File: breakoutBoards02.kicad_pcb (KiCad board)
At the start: 2 copper layers, 50 x 50 mm, 45 parts, among them J1 USB_2, M1 Mounting Hole (0.125"), M2 Mounting Hole (0.125"), M3 Mounting Hole (0.125"), M4 Mounting Hole (0.125"), P1 CONN_12, P2 CONN_12, U1 EEPROM_SPI, U2 FT232H, X1 12MHz

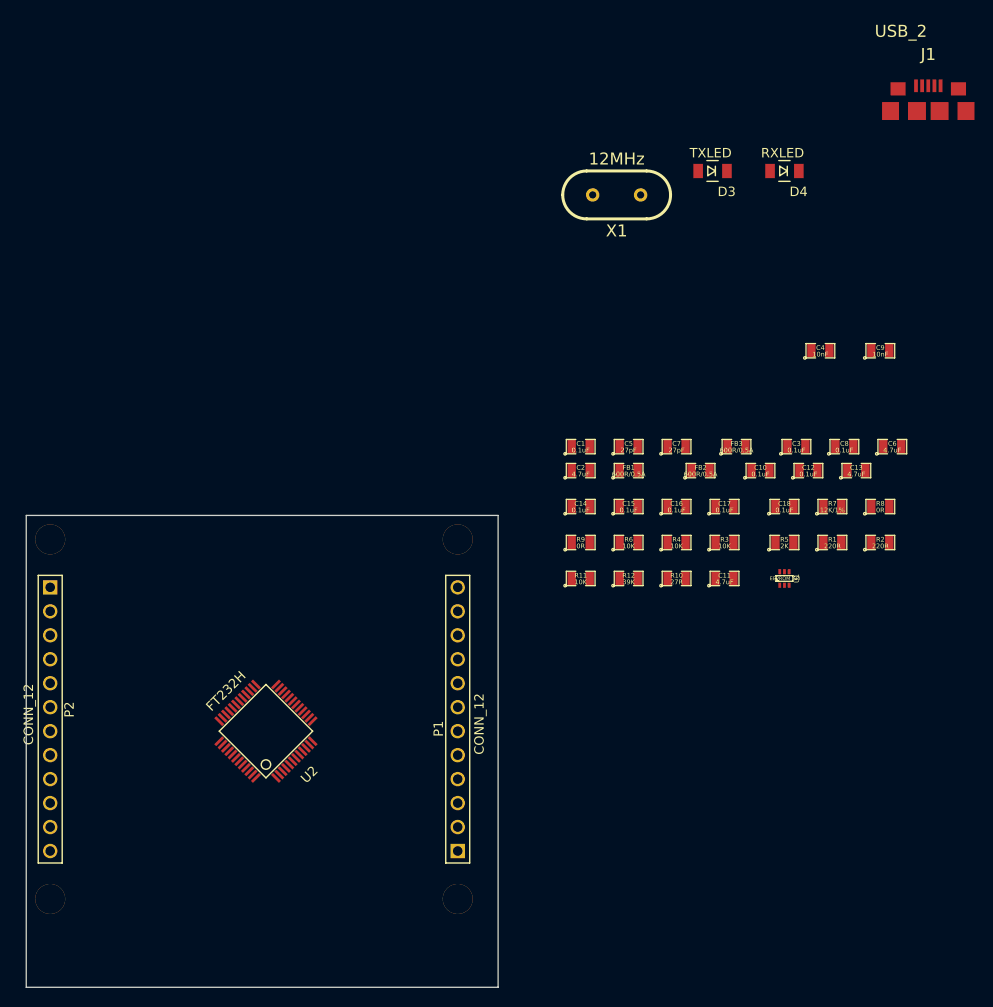
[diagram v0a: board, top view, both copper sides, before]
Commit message: initial layout
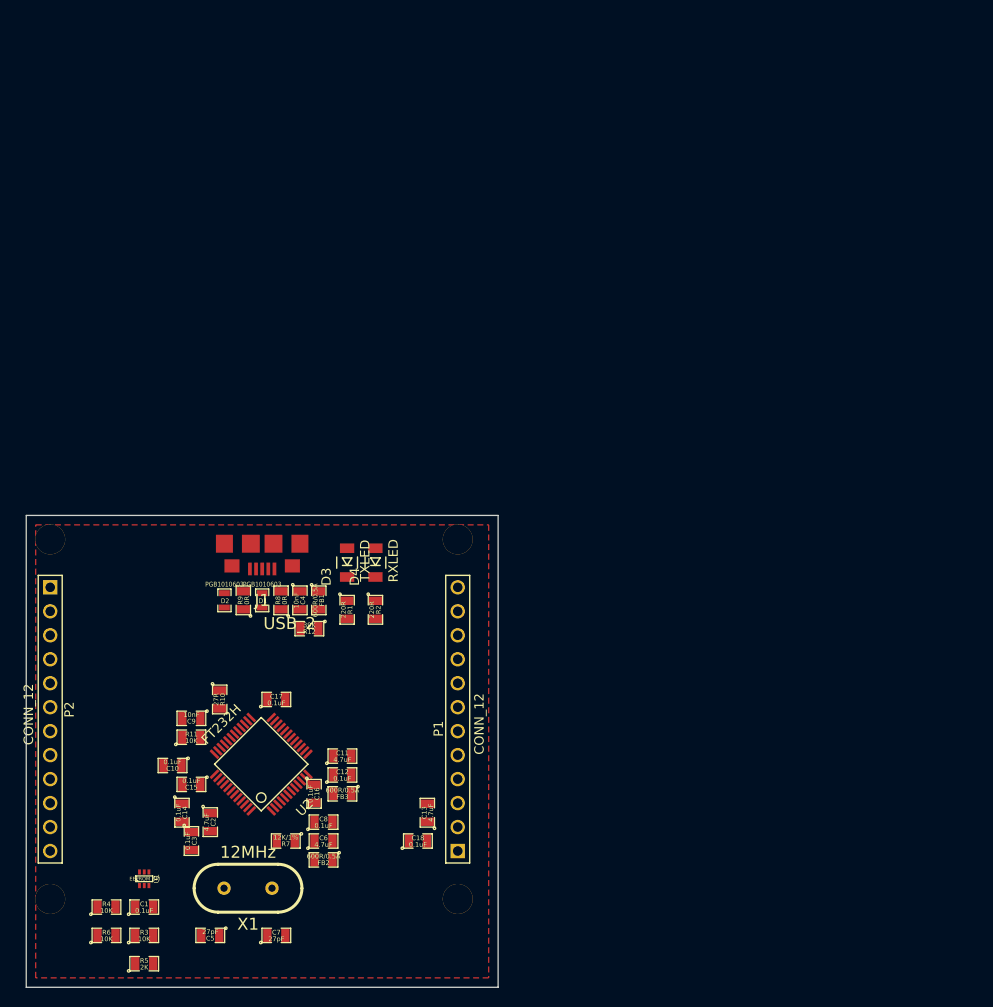
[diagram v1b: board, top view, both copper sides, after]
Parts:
- added D1: PGB1010603, SM0603_Resistor, F.Cu at (125.0, 109.0)
- added D2: PGB1010603, SM0603_Resistor, F.Cu at (121.0, 109.0)
- moved J1 84.2 mm to (125.0, 103.0), turned to 180 degrees
- moved X1 83.2 mm to (123.5, 139.5)
- moved C9 82.7 mm to (117.5, 121.5), turned to 180 degrees
- moved R5 81.2 mm to (112.5, 147.5)
- moved C3 76.5 mm to (117.5, 134.5), turned to 270 degrees
- moved U1 74.9 mm to (112.5, 138.5)
- moved R3 74.3 mm to (112.5, 144.5)
- moved C6 73.3 mm to (131.5, 134.5)
- moved R4 71.7 mm to (108.5, 141.5)
- moved C10 69.7 mm to (115.5, 126.5), turned to 180 degrees
- moved R6 69.2 mm to (108.5, 144.5)
- moved C5 68.2 mm to (119.5, 144.5), turned to 180 degrees
- moved C8 68.0 mm to (131.5, 132.5)
- moved R7 67.9 mm to (127.5, 134.5), turned to 180 degrees
- moved C1 67.2 mm to (112.5, 141.5)
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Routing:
- added copper zone on F.Cu, net GND

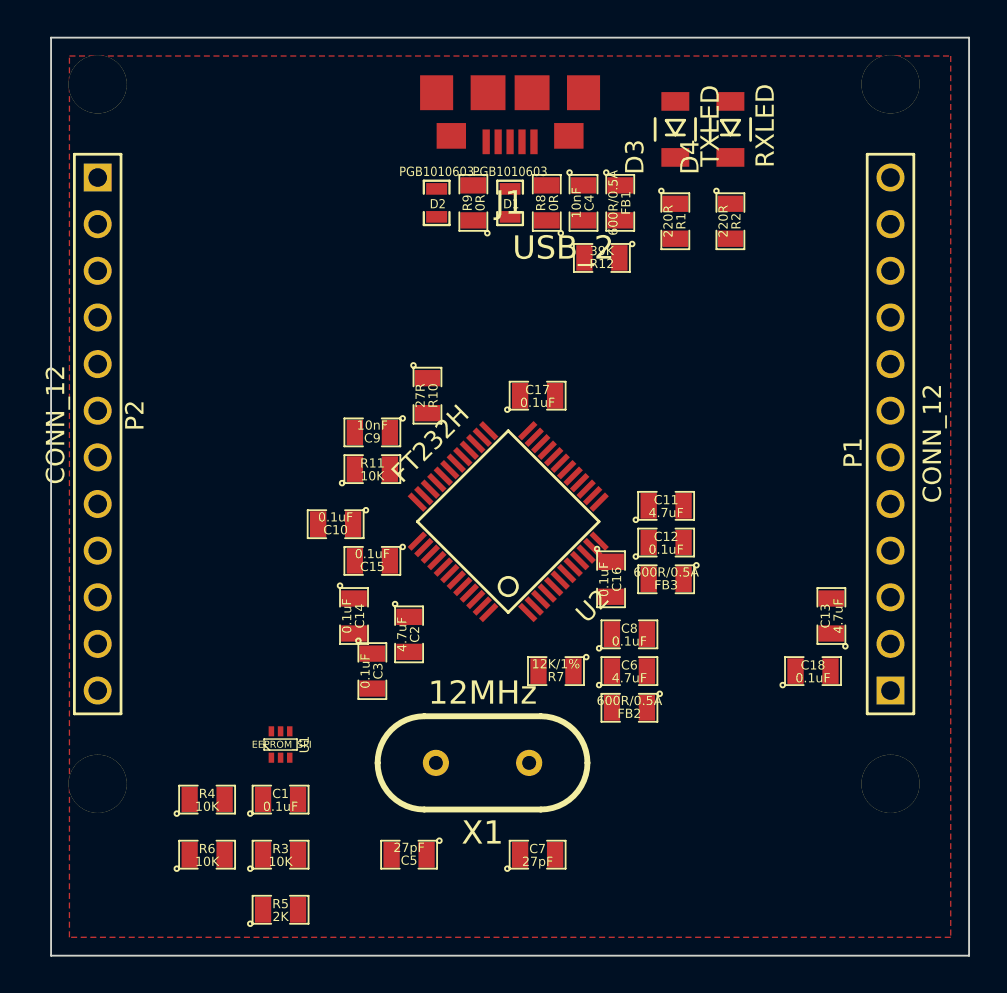
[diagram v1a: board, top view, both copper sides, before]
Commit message: boards
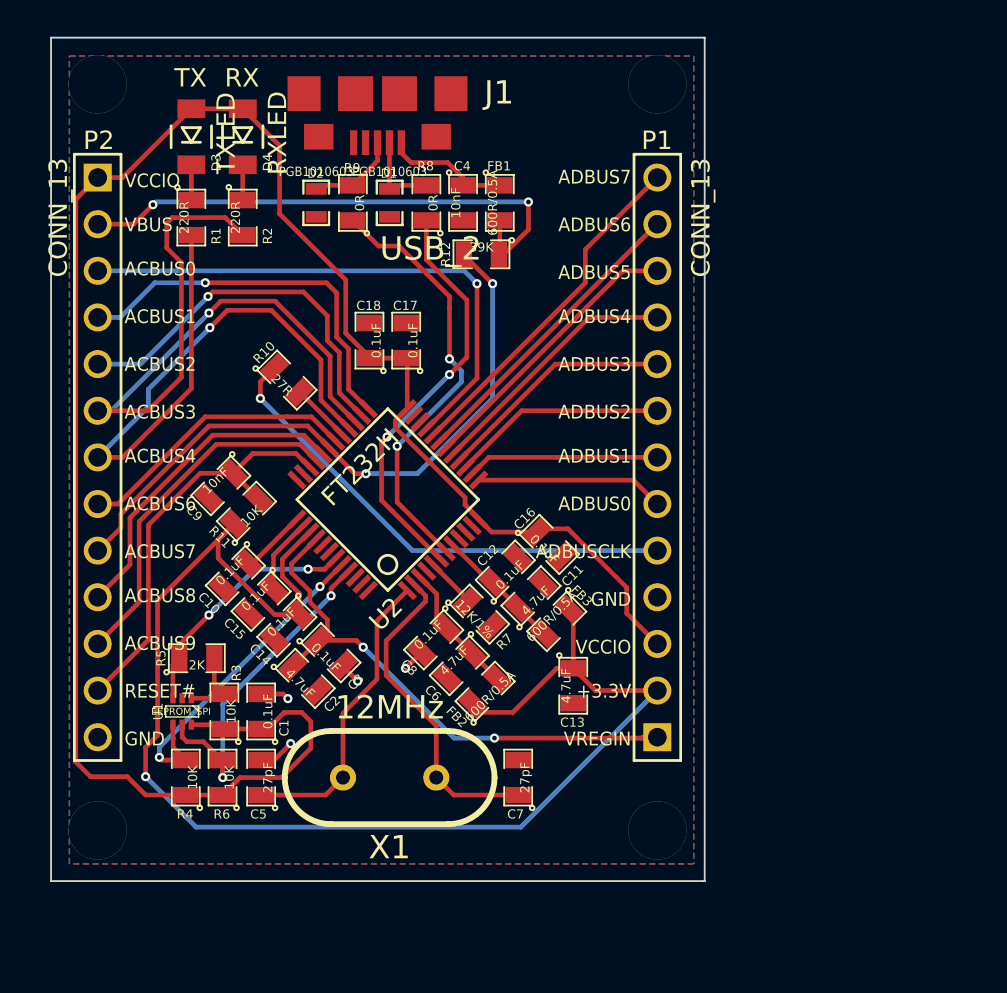
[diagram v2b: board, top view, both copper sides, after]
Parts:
- P1, P2: value CONN_12 -> CONN_13; footprint PIN_ARRAY_12X1 -> PIN_ARRAY_13X1
- moved C18 30.1 mm to (117.3, 116.5), turned to 90 degrees
- moved D4 26.6 mm to (110.4, 105.4)
- moved R2 26.6 mm to (110.4, 109.8)
- moved D3 26.4 mm to (107.6, 105.4)
- moved R1 26.4 mm to (107.6, 109.8)
- moved C13 14.6 mm to (128.4, 135.3), turned to 270 degrees
- moved R5 14.4 mm to (107.9, 133.8)
- moved M1 13.0 mm to (133.0, 143.2)
- moved P1 13.0 mm to (133.0, 125.4)
- moved M4 12.7 mm to (133.0, 102.5)
- moved C8 10.7 mm to (120.8, 132.8), turned to 225 degrees
- moved C6 9.26 mm to (122.2, 134.2), turned to 225 degrees
- moved C5 9.09 mm to (111.4, 140.3), turned to 90 degrees
- moved C12 8.89 mm to (124.7, 129.0), turned to 45 degrees
- moved C11 8.84 mm to (126.1, 130.4), turned to 45 degrees
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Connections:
- net N-0000024 renamed /ADBUS3
- net N-0000025 renamed /ADBUS2
- net N-0000026 renamed /ADBUS1
- net N-0000027 renamed /ADBUS0
- net N-0000029 renamed /ADBUS4
- net N-0000030 renamed /ACBUS8
- net N-0000033 renamed /ACBUS9
- net N-0000034 renamed /ACBUS6
- P1 pad 1: VBUS -> VREGIN
- P1 pad 11: N-0000040 (its old number) -> /ADBUS5
- P1 pad 12: N-0000039 (its old number) -> /ADBUS6
- P1 pad 2: VREGIN -> +3.3V
- P1 pad 3: +3.3V -> VCCIO
- P1 pad 4: VCCIO -> GND
- P1 pad 5: GND -> /ADBUSCLK
- P2 pad 1: N-0000038 (its old number) -> VCCIO
- P2 pad 2: N-0000037 (its old number) -> VBUS
- P2 pad 3: N-0000036 -> /ACBUS0
- P2 pad 4: N-0000035 -> /ACBUS1
- P2 pad 5: /RXLED# -> /ACBUS2
- P2 pad 6: /TXLED# -> /RXLED#
- P2 pad 7: N-0000021 -> /TXLED#
- P2 pad 9: N-000001 (its old number) -> /ACBUS7
- R10 pad 1: N-0000021 -> /ADBUSCLK
- R12 pad 2: N-000001 (its old number) -> /ACBUS7
- R8 pad 1: N-000009 (its old number) -> /USBDM
- R9 pad 1: N-000008 (its old number) -> /USBDP
- U2 pad 18: N-0000040 (its old number) -> /ADBUS5
- U2 pad 19: N-0000039 (its old number) -> /ADBUS6
- U2 pad 20: N-0000038 (its old number) -> /ADBUS7
- U2 pad 21: N-0000037 (its old number) -> /ACBUS0
- U2 pad 25: N-0000036 -> /ACBUS1
- U2 pad 26: N-0000035 -> /ACBUS2
- U2 pad 31: N-000001 (its old number) -> /ACBUS7
- U2 pad 6: N-000009 (its old number) -> /USBDM
- U2 pad 7: N-000008 (its old number) -> /USBDP
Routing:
- net VCCIO: track 0.00 -> 107.9 mm
- net +3.3V: track 0.00 -> 76.4 mm, vias 0 -> 1
- net /RXLED#: track 0.00 -> 39.2 mm, vias 0 -> 1
- net /TXLED#: track 0.00 -> 36.5 mm, vias 0 -> 1
- net /ACBUS7: track 0.00 -> 36.0 mm, vias 0 -> 2
- net /ACBUS0: track 0.00 -> 30.0 mm, vias 0 -> 1
- net VREGIN: track 0.00 -> 29.8 mm, vias 0 -> 2
- net VBUS: track 0.00 -> 29.5 mm, vias 0 -> 2
- net /ADBUSCLK: track 0.00 -> 27.1 mm, vias 0 -> 1
- net /USBDP: track 0.00 -> 23.7 mm, vias 0 -> 2
- net /RESET#: track 0.00 -> 22.9 mm
- net /USBDM: track 0.00 -> 22.6 mm, vias 0 -> 2
- net /ACBUS1: track 0.00 -> 21.1 mm, vias 0 -> 1
- net /ACBUS2: track 0.00 -> 20.9 mm, vias 0 -> 1
- net /ACBUS9: track 0.00 -> 19.4 mm
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- added copper zone on B.Cu, net GND
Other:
- board size 50 x 50 mm -> 35.6 x 45.9 mm
- net class Default: clearance 0.254 -> 0.2032; via_dia 0.889 -> 0.5; via_drill 0.635 -> 0.35
- rule trace_clearance: 0.254 -> 0.2032
- rule trace_min: 0.254 -> 0.008
- rule via_min_drill: 0.508 -> 0.3
- rule via_min_size: 0.889 -> 0.035
- board text added: "+3.3V"
- board text added: "ACBUS0"
- board text added: "ACBUS1"
- board text added: "ACBUS2"
- board text added: "ACBUS3"
- board text added: "ACBUS4"
- board text added: "ACBUS6"
- board text added: "ACBUS7"
- board text added: "ACBUS8"
- board text added: "ACBUS9"
- board text added: "ADBUS0"
- board text added: "ADBUS1"
- board text added: "ADBUS2"
- board text added: "ADBUS3"
- board text added: "ADBUS4"
- board text added: "ADBUS5"
- board text added: "ADBUS6"
- board text added: "ADBUS7"
- board text added: "ADBUSCLK"
- board text added: "GND"
- board text added: "RESET#"
- board text added: "RX"
- board text added: "TX"
- board text added: "VBUS"
- board text added: "VCCIO"
- board text added: "VREGIN"
